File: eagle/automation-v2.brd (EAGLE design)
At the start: 65.8 x 104.1 mm, 96 parts, among them IC1 MEGA48/88/168-AU, IC2 DS2482-100S, IC3 DS2482-100S, IC4 78L33, K1 SRD-05VDC-SL-C, K2 SRD-05VDC-SL-C, K3 SRD-05VDC-SL-C, K4 SRD-05VDC-SL-C, Q1 BSS123, Q2 BSS123, Q3 BSS123, Q4 BSS123, X1 OPI-ZERO

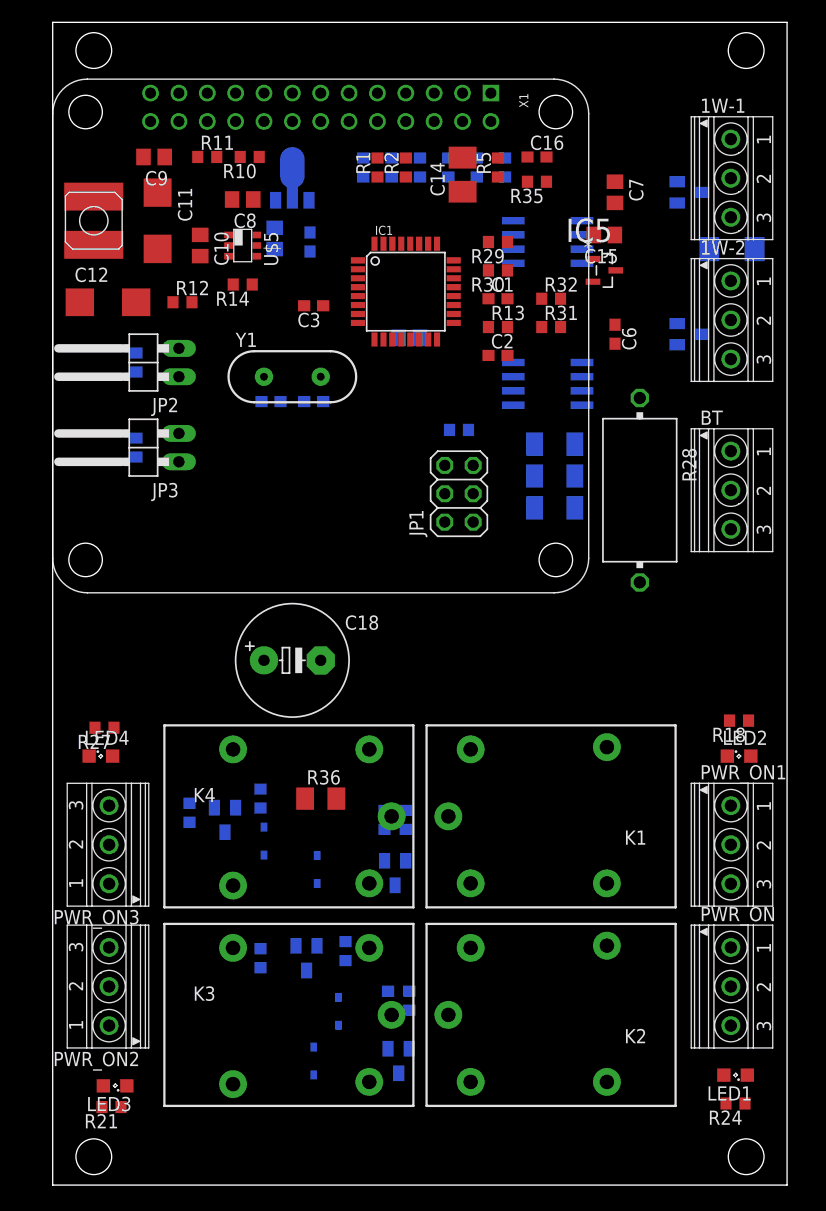
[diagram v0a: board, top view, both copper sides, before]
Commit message: Initial PCB trace
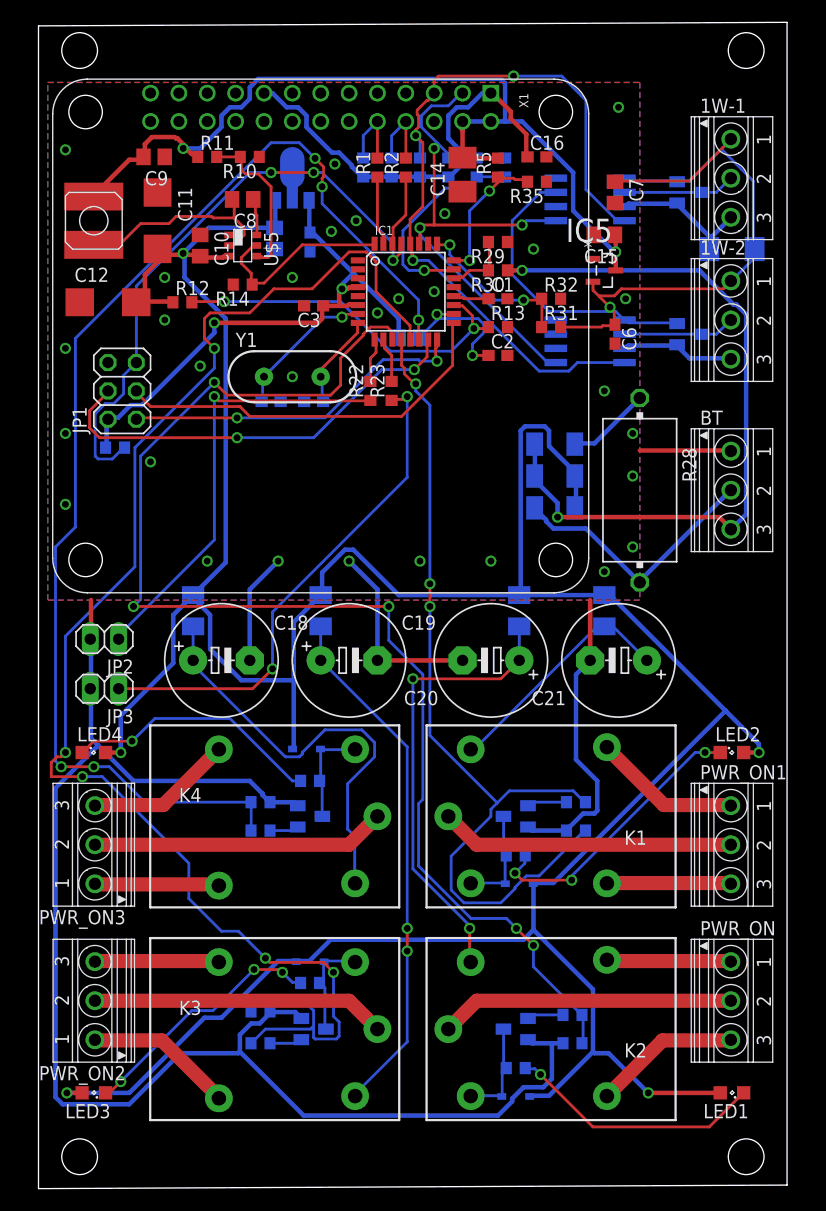
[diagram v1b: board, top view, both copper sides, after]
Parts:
- added C19, C20, C21: (no value), rcl:E5-10,5
- added R37, R38, R39: (no value), rcl:M1206
- JP2, JP3: device pinhead:1X02/90 -> pinhead:1X02
- moved JP1 31.5 mm to (6.35, 17.8)
- moved R8 30.8 mm to (5.71, 12.7)
- moved JP2 24.9 mm to (4.76, -4.45), turned to 180 degrees
- moved R23 23.4 mm to (30.5, 17.8), flipped to the top
- moved R18 23.4 mm to (41.6, -23.8), flipped to the bottom
- moved JP3 21.8 mm to (4.76, -8.89), turned to 180 degrees
- moved R22 21.1 mm to (28.6, 17.8), flipped to the top
- moved R21 21.0 mm to (23.2, -35.2), flipped to the bottom, turned to 0 degrees
- moved R36 20.3 mm to (12.7, -1.91), flipped to the bottom, turned to 270 degrees
- moved R24 19.9 mm to (41.6, -42.9), flipped to the bottom
- moved R27 19.0 mm to (23.2, -17.1), flipped to the bottom, turned to 0 degrees
- moved D2 18.4 mm to (41.6, -45.4), turned to 0 degrees
- moved D1 18.1 mm to (41.9, -26.4), turned to 0 degrees
- moved R16 17.2 mm to (47.0, -19.1), turned to 180 degrees
- moved R9 16.6 mm to (46.7, -38.1), turned to 180 degrees
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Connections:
- new net N$14: C19.+, K3.A2, R37.2
- new net N$63: C20.+, K2.A2, R38.1
- new net N$66: C21.+, K1.A2, R39.1
- net 12V: now also R37.1, R38.2, R39.2; no longer K1.A2, K2.A2, K3.A2
- net GND: now also C19.-, C20.-, C21.-
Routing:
- net 12V: track 0.00 -> 296.1 mm, vias 0 -> 5
- net GND: track 0.00 -> 218.0 mm, vias 0 -> 30
- net N$46: track 0.00 -> 131.9 mm, vias 0 -> 5
- net N$23: track 0.00 -> 115.9 mm, vias 0 -> 5
- net N$53: track 0.00 -> 109.7 mm, vias 0 -> 5
- net VDD: track 0.00 -> 86.0 mm, vias 0 -> 1
- net Z5V: track 0.00 -> 79.9 mm, vias 0 -> 2
- net N$24: track 0.00 -> 78.7 mm, vias 0 -> 3
- net N$2: track 0.00 -> 70.6 mm, vias 0 -> 3
- net N$12: track 0.00 -> 66.2 mm, vias 0 -> 2
- net N$13: track 0.00 -> 53.5 mm, vias 0 -> 3
- net VCC: track 0.00 -> 51.8 mm, vias 0 -> 2
- net N$1: track 0.00 -> 48.2 mm, vias 0 -> 3
- net N$14: track 0.00 -> 47.2 mm, vias 0 -> 2
- net N$40: track 0.00 -> 45.5 mm, vias 0 -> 2
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- added copper zone on layer 1, net GND
- added copper zone on layer 16, net GND
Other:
- board size 65.8 x 104.1 mm -> 67 x 104.4 mm
